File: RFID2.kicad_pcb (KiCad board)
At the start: 2 copper layers, 28 parts, among them J1 USB_B_Micro, J2 Conn_01x01_Pin, J3 Conn_01x01_Pin, Q1 BS170, Q2 BC547, U1 ATtiny13-20M, U3 LM358, U4 LM358

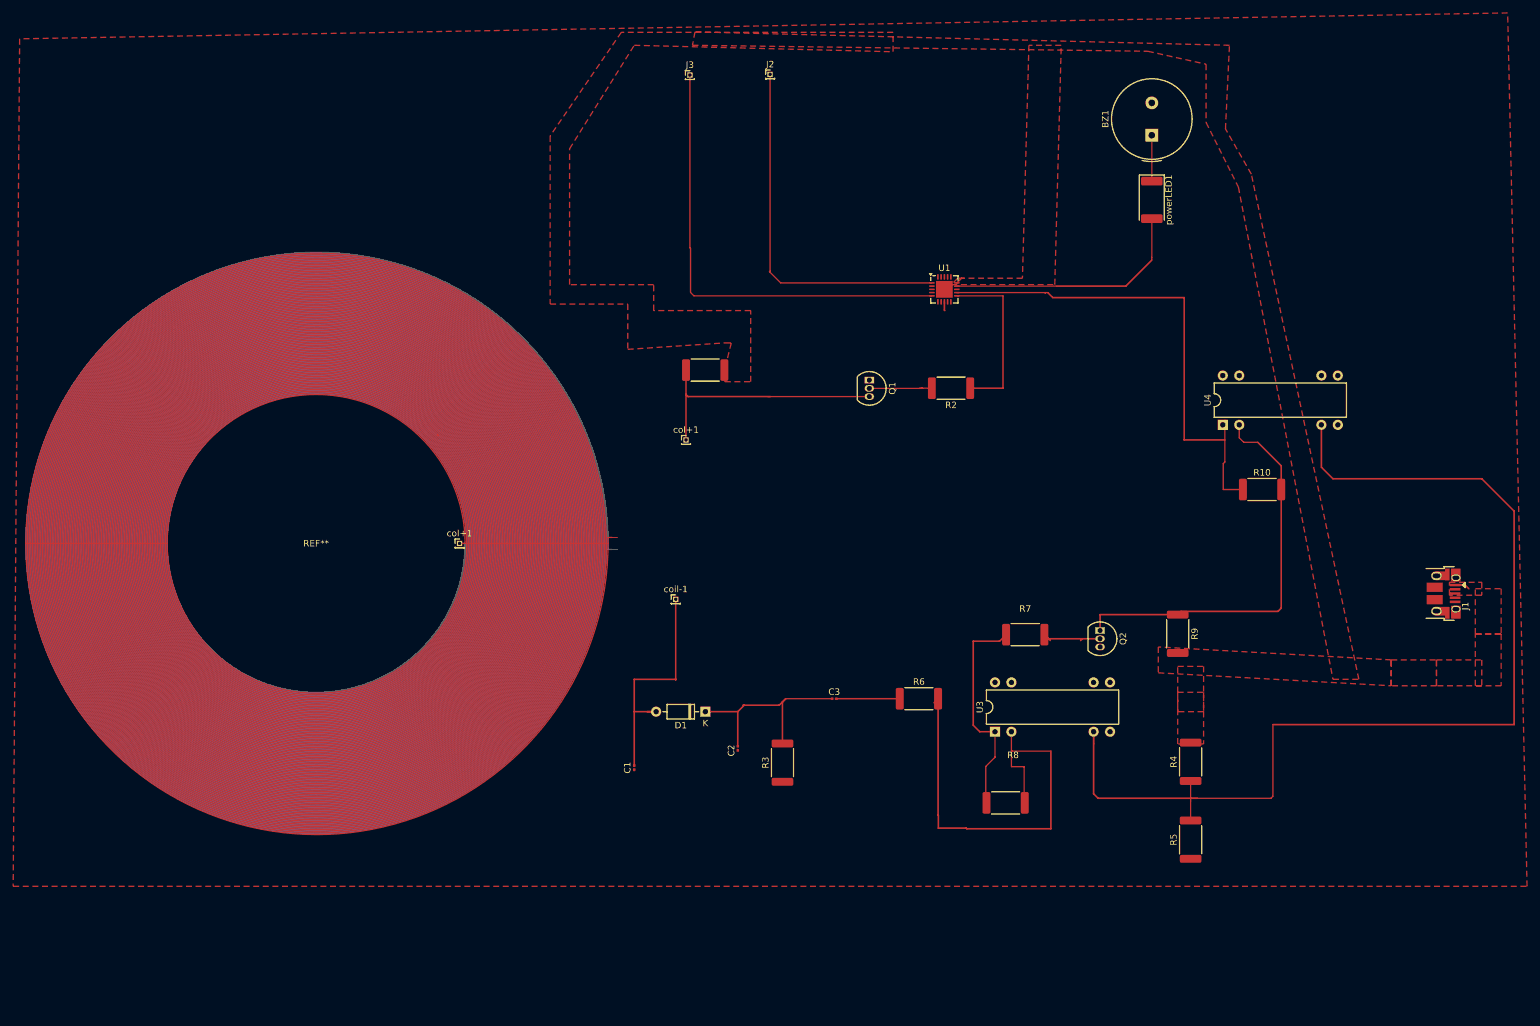
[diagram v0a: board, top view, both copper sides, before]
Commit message: pcb
updated
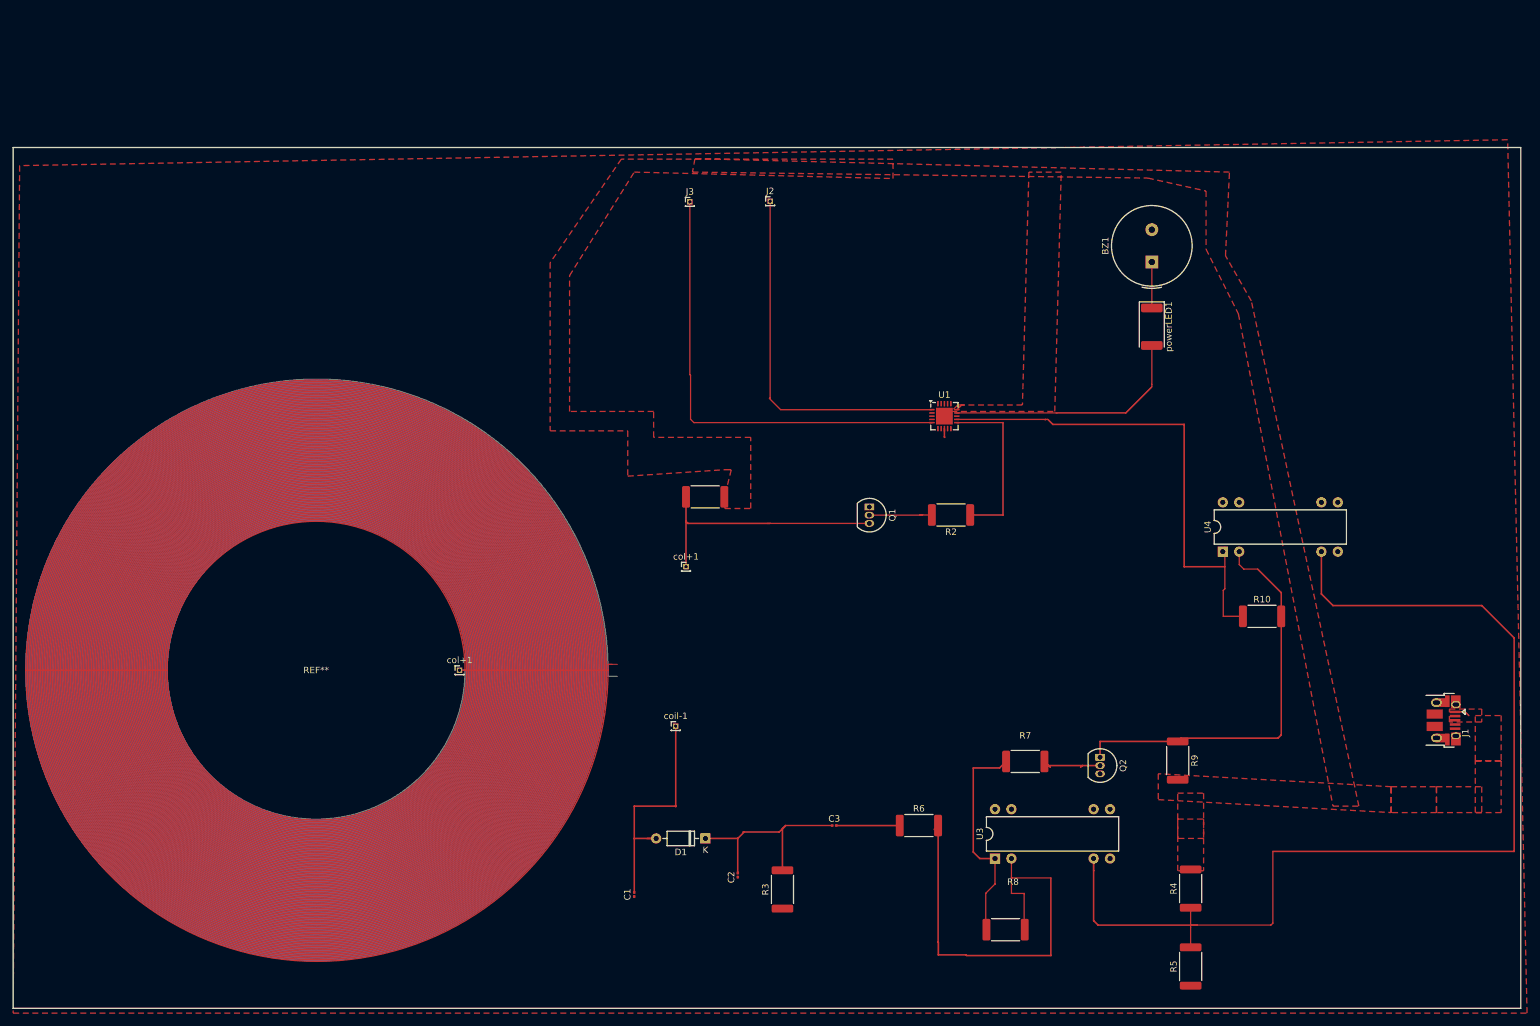
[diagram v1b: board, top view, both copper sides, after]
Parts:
- moved J1 19.6 mm to (257.1, 119.4)
- moved Q2 19.6 mm to (204.0, 125.1)
- moved R7 19.6 mm to (192.4, 125.7)
- moved BZ1 19.6 mm to (212.0, 48.5)
- moved J2 19.6 mm to (153.0, 39.1)
- moved J3 19.6 mm to (140.6, 39.2)
- moved U1 19.6 mm to (179.9, 72.3)
- moved powerLED1 19.6 mm to (212.0, 58.5)
- moved C1 19.6 mm to (132.0, 146.3)
- moved C2 19.6 mm to (148.0, 143.3)
- moved C3 19.6 mm to (162.9, 135.6)
- moved D1 19.6 mm to (143.0, 137.6)
- moved Q1 19.6 mm to (168.3, 86.4)
- moved R1 19.6 mm to (143.0, 84.8)
- moved R10 19.6 mm to (229.0, 103.3)
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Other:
- board outline added: 233 x 133.1 mm
